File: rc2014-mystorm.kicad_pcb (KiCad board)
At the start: 2 copper layers, 100 x 50 mm, 15 parts, among them J1 CONN_02X06, J2 CONN_02X06, J3 CONN_02X06, J4 CONN_02X06, J6 CONN_02X06, J7 CONN_01X06, P1 RC2014 BUS, U1 SN74LVCC3245A, U2 SN74LVCC3245A, U3 SN74LVCC3245A, U4 SN74LVCC3245A

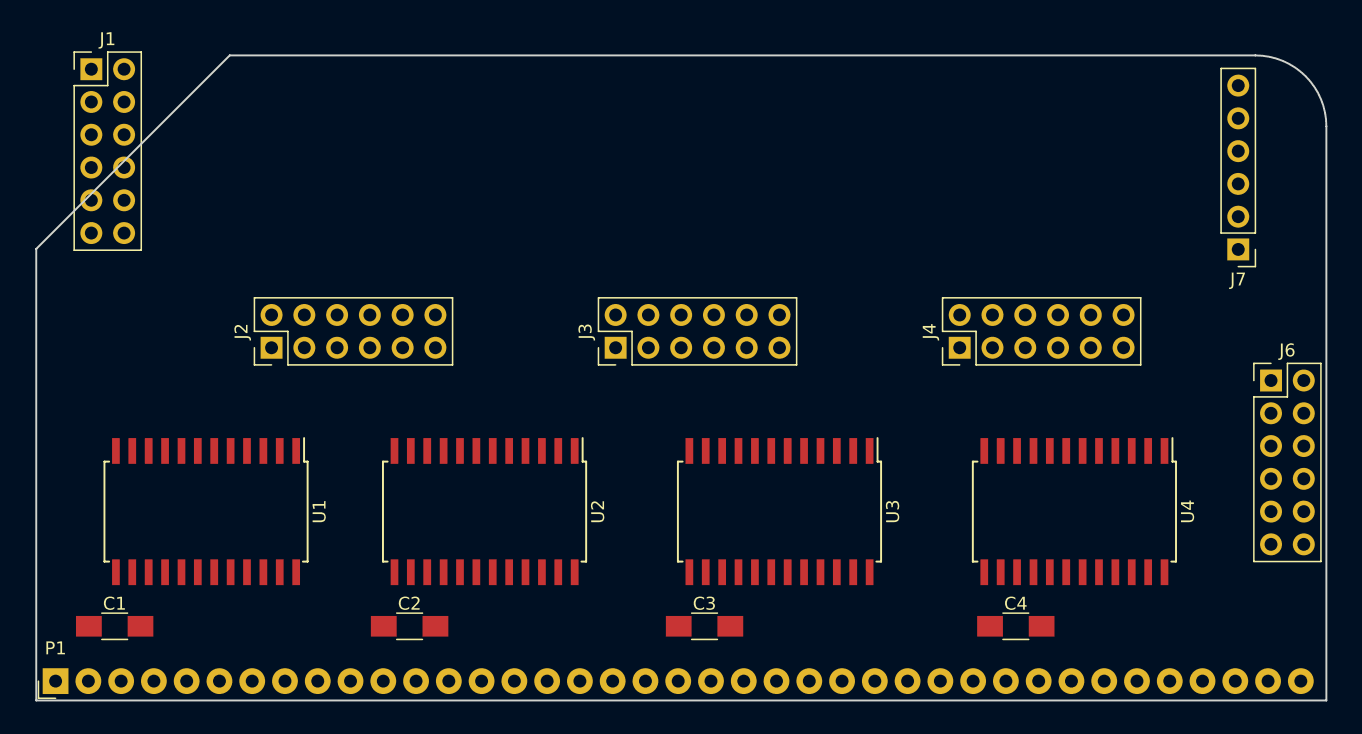
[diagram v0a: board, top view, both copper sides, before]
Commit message: further SMT WIP
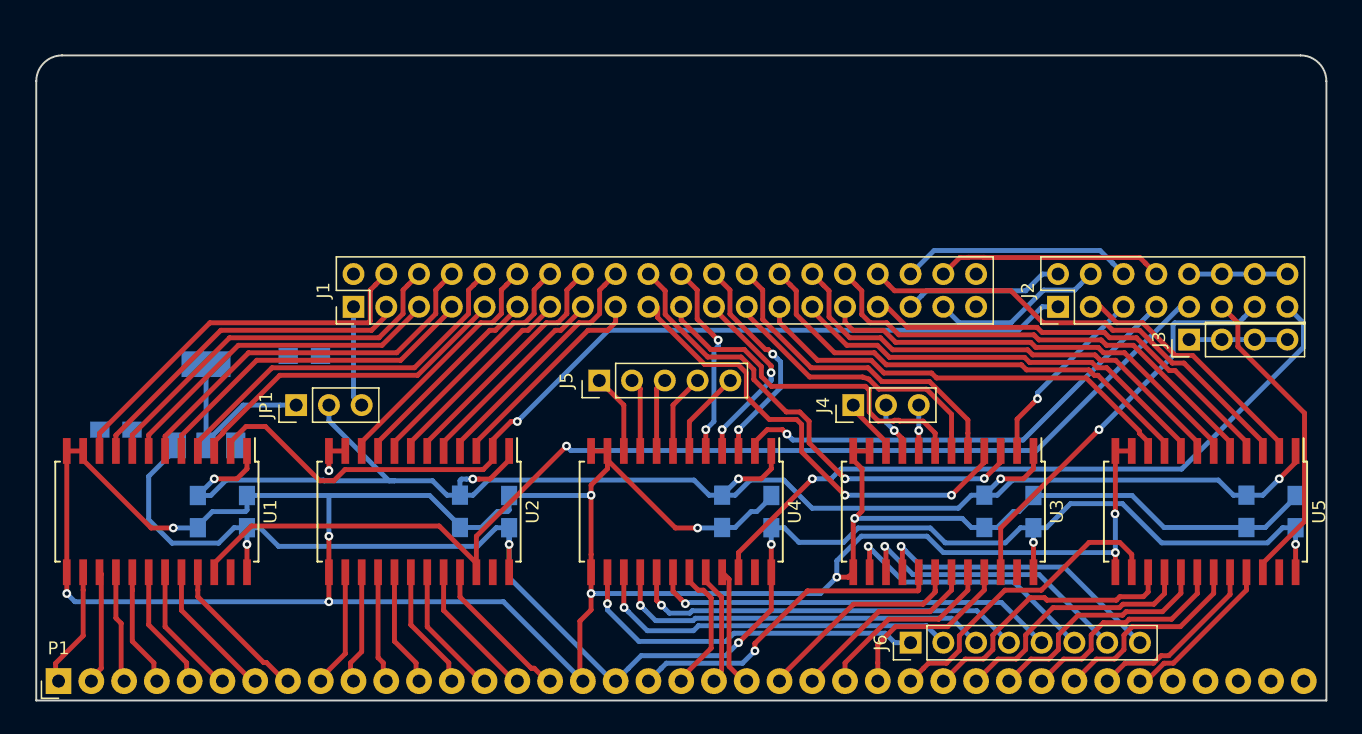
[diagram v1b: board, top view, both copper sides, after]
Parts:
- removed J7: CONN_01X06, Pin_Headers:Pin_Header_Straight_1x06_Pitch2.54mm
- added C10: C, Capacitors_SMD:C_0805_HandSoldering, B.Cu at (117.5, 149.9)
- added C11: C, Capacitors_SMD:C_0805_HandSoldering, B.Cu at (137.8, 149.9)
- added C12: C, Capacitors_SMD:C_0805_HandSoldering, B.Cu at (158.1, 149.9)
- added C5: C, Capacitors_SMD:C_0805_HandSoldering, B.Cu at (113.7, 149.8)
- added C6: C, Capacitors_SMD:C_0805_HandSoldering, B.Cu at (134.0, 149.8)
- added C7: C, Capacitors_SMD:C_0805_HandSoldering, B.Cu at (154.3, 149.8)
- added C8: C, Capacitors_SMD:C_0805_HandSoldering, B.Cu at (76.8, 149.9)
- added C9: C, Capacitors_SMD:C_0805_HandSoldering, B.Cu at (97.2, 149.9)
- added J5: Conn_01x05, Pin_Headers:Pin_Header_Straight_1x05_Pitch2.54mm, F.Cu at (104.1, 139.7)
- added JP1: Ext Power, Pin_Headers:Pin_Header_Straight_1x03_Pitch2.54mm, F.Cu at (80.6, 141.6)
- added U5: SN74LVCC3245A, Housings_SOIC:SOIC-24W_7.5x15.4mm_Pitch1.27mm, F.Cu at (151.1, 149.9)
- added U6: LM1117-3.3, TO_SOT_Packages_SMD:SOT-223-3_TabPin2, B.Cu at (73.7, 141.6)
- C1, C2: value C -> CP_Small; footprint Capacitors_SMD:C_1206_HandSoldering -> Capacitors_SMD:C_0805_HandSoldering; moved to B.Cu
- C3, C4: footprint Capacitors_SMD:C_1206_HandSoldering -> Capacitors_SMD:C_0805_HandSoldering; moved to B.Cu
- J1: value CONN_02X06 -> FPGA connection; footprint Pin_Headers:Pin_Header_Straight_2x06_Pitch2.54mm -> Pin_Headers:Pin_Header_Straight_2x20_Pitch2.54mm
- J2: value CONN_02X06 -> Config; footprint Pin_Headers:Pin_Header_Straight_2x06_Pitch2.54mm -> Pin_Headers:Pin_Header_Straight_2x08_Pitch2.54mm
- J3: value CONN_02X06 -> Conn_01x05; footprint Pin_Headers:Pin_Header_Straight_2x06_Pitch2.54mm -> Pin_Headers:Pin_Header_Straight_1x04_Pitch2.54mm
- J4: value CONN_02X06 -> Conn_01x03; footprint Pin_Headers:Pin_Header_Straight_2x06_Pitch2.54mm -> Pin_Headers:Pin_Header_Straight_1x03_Pitch2.54mm
- J6: value CONN_02X06 -> Extra; footprint Pin_Headers:Pin_Header_Straight_2x06_Pitch2.54mm -> Pin_Headers:Pin_Header_Straight_1x08_Pitch2.54mm
- moved J2 61.0 mm to (139.7, 134.0)
- moved J3 44.5 mm to (149.9, 136.5)
- moved C4 44.0 mm to (93.3, 149.8), turned to 270 degrees
- moved C3 40.3 mm to (73.0, 149.9), turned to 270 degrees
- moved J6 34.5 mm to (128.3, 160.0), turned to 90 degrees
- moved U4 30.5 mm to (110.5, 149.9)
- moved J1 27.4 mm to (85.1, 134.0), turned to 90 degrees
- moved C2 22.5 mm to (81.3, 137.8)
- moved C1 15.2 mm to (66.7, 143.5)
- moved U3 12.7 mm to (130.8, 149.9)
- moved J4 9.38 mm to (123.8, 141.6)
- moved U2 5.08 mm to (90.2, 149.9)
- moved U1 3.81 mm to (69.8, 149.9)
- moved P1 0.23 mm to (62.2, 163.0)
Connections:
- C1 pad 1: (no net) -> +5V
- C2 pad 1: (no net) -> Net-(C2-Pad1)
- C2 pad 2: (no net) -> GND
- C3 pad 1: (no net) -> +3V3
- C3 pad 2: (no net) -> GND
- C4 pad 1: (no net) -> +3V3
- C4 pad 2: (no net) -> GND
- J1 pad 1: GND -> /FPGA_VCC
- J1 pad 10: /A11LV -> /A9LV
- J1 pad 11: /A8LV -> /A6LV
- J1 pad 12: /A9LV -> /A7LV
- J1 pad 3: +3V3 -> /A14LV
- J1 pad 4: +3V3 -> /A15LV
- J1 pad 5: /A14LV -> /A12LV
- J1 pad 6: /A15LV -> /A13LV
- J1 pad 7: /A12LV -> /A10LV
- J1 pad 8: /A13LV -> /A11LV
- J1 pad 9: /A10LV -> /A8LV
- J2 pad 1: +3V3 -> /ADDR_DIR
- J2 pad 10: /A3LV -> GND
- J2 pad 11: /A0LV -> /DATA_OE
- J2 pad 12: /A1LV -> GND
- J2 pad 2: +3V3 -> /GPIO1
- J2 pad 3: GND -> /DATA_DIR
- J2 pad 4: GND -> /GPIO2
- J2 pad 5: /A6LV -> /SIG_DIR
- J2 pad 6: /A7LV -> /GPIO3
- J2 pad 7: /A4LV -> /SIG2_DIR
- J2 pad 8: /A5LV -> /GPIO4
- J2 pad 9: /A2LV -> /ADDR_OE
- J3 pad 3: GND -> +3V3
- J3 pad 4: GND -> +3V3
- J4 pad 1: /ADDR_DIR -> /EX3LV
- J4 pad 2: (no net) -> /EX2LV
- J4 pad 3: /DATA_DIR -> /EX1LV
- J6 pad 1: +3V3 -> /EX8
- J6 pad 2: +3V3 -> /EX7
- J6 pad 3: GND -> /EX6
- J6 pad 4: GND -> /EX5
- J6 pad 5: /D0LV -> /EX4
- J6 pad 6: /D1LV -> /EX3
- J6 pad 7: /D2LV -> /EX2
- J6 pad 8: /D3LV -> /EX1
- U1 pad 10: /A8LV -> /A15LV
- U1 pad 3: /A15LV -> /A8LV
- U1 pad 4: /A14LV -> /A9LV
- U1 pad 5: /A13LV -> /A10LV
- U1 pad 6: /A12LV -> /A11LV
- U1 pad 7: /A11LV -> /A12LV
- U1 pad 8: /A10LV -> /A13LV
- U1 pad 9: /A9LV -> /A14LV
- U2 pad 10: /A0LV -> /A7LV
- U2 pad 3: /A7LV -> /A0LV
- U2 pad 4: /A6LV -> /A1LV
- U2 pad 5: /A5LV -> /A2LV
- U2 pad 6: /A4LV -> /A3LV
- U2 pad 7: /A3LV -> /A4LV
- U2 pad 8: /A2LV -> /A5LV
- U2 pad 9: /A1LV -> /A6LV
- U3 pad 10: //IORQLV -> /EX3LV
- U3 pad 14: /M1 -> /EX3
- U3 pad 15: //RESET -> /EX2
- U3 pad 16: /CLK -> /EX1
- U3 pad 17: /INT -> /M1
- U3 pad 3: /M1LV -> //IORQLV
- U3 pad 4: //RESETLV -> //RDLV
- U3 pad 5: /CLKLV -> //WRLV
- U3 pad 6: /INTLV -> /MREQLV
- U3 pad 7: /MREQLV -> /M1LV
- U3 pad 8: //WRLV -> /EX1LV
- U3 pad 9: //RDLV -> /EX2LV
- U4 pad 10: /D7LV -> /EX8LV
- U4 pad 14: /D0 -> /EX8
- U4 pad 15: /D1 -> /EX7
- U4 pad 16: /D2 -> /EX6
- U4 pad 17: /D3 -> /EX5
- U4 pad 18: /D4 -> /EX4
- U4 pad 19: /D5 -> //RESET
- U4 pad 2: /DATA_DIR -> /SIG2_DIR
- U4 pad 20: /D6 -> /CLK
- U4 pad 21: /D7 -> /INT
- U4 pad 22: /DATA_OE -> /SIG2_OE
- U4 pad 3: /D0LV -> /INTLV
- U4 pad 4: /D1LV -> /CLKLV
- U4 pad 5: /D2LV -> //RESETLV
- U4 pad 6: /D3LV -> /EX4LV
- U4 pad 7: /D4LV -> /EX5LV
- U4 pad 8: /D5LV -> /EX6LV
- U4 pad 9: /D6LV -> /EX7LV
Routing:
- net GND: track 0.00 -> 263.6 mm, vias 0 -> 12
- net +5V: track 0.00 -> 132.2 mm, vias 0 -> 6
- net +3V3: track 0.00 -> 132.1 mm, vias 0 -> 5
- net /ADDR_OE: track 0.00 -> 89.8 mm, vias 0 -> 1
- net /ADDR_DIR: track 0.00 -> 74.3 mm, vias 0 -> 1
- net /SIG2_OE: track 0.00 -> 55.6 mm, vias 0 -> 1
- net //IORQLV: track 0.00 -> 38.5 mm, vias 0 -> 2
- net /D3LV: track 0.00 -> 37.1 mm
- net /D1LV: track 0.00 -> 37.0 mm
- net /D5LV: track 0.00 -> 37.0 mm
- net /SIG2_DIR: track 0.00 -> 36.8 mm, vias 0 -> 1
- net //RDLV: track 0.00 -> 36.8 mm, vias 0 -> 2
- net /D7LV: track 0.00 -> 35.9 mm
- net /D0LV: track 0.00 -> 34.4 mm
- net /D4LV: track 0.00 -> 34.3 mm
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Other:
- outline, holes or cut-outs redrawn
- net class Default: clearance 0.254 -> 0.2
- rule trace_clearance: 0.254 -> 0.2
- board text added: "A15"
- board text added: "github.com/electrified/rc2014-fpga"
- board text removed: "github.com/electrified/rc2014-ym2149"

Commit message: WIP
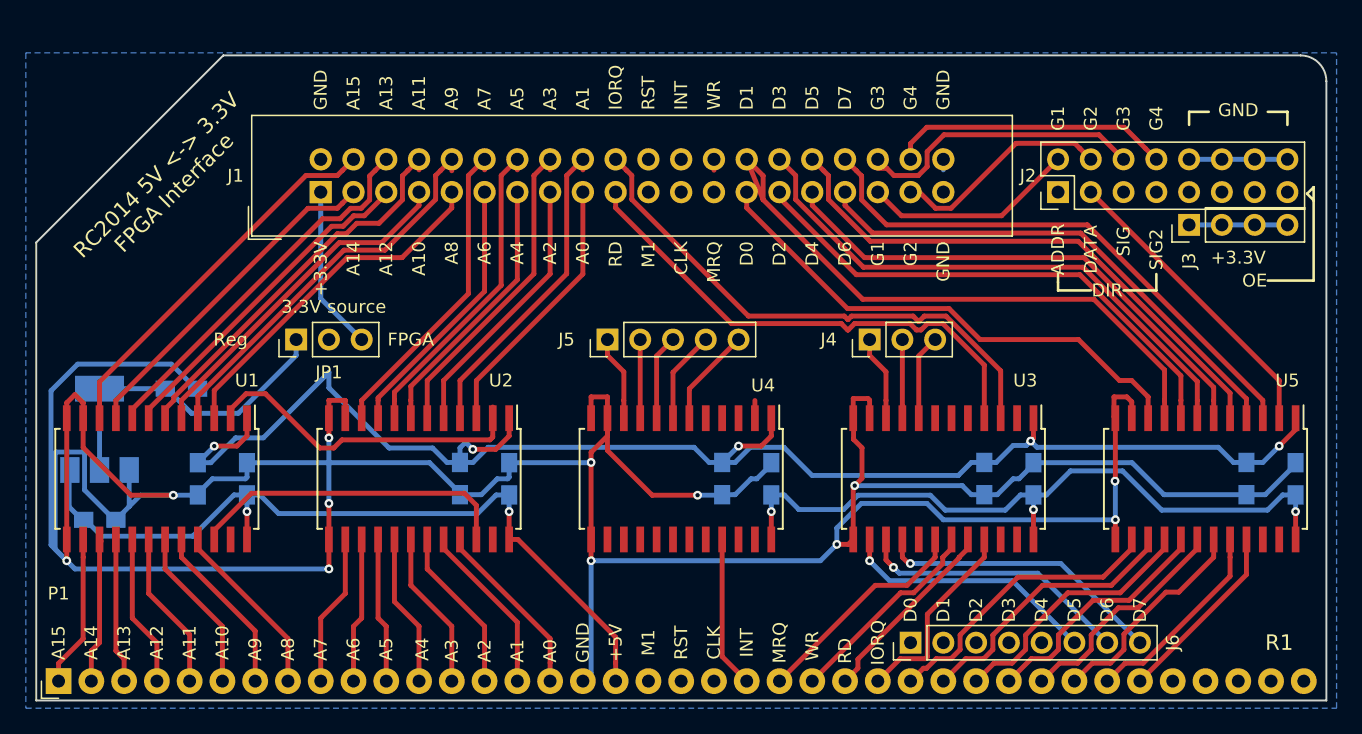
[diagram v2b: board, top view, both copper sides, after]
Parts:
- added REF***: OSHW-Logo_7.5x8mm_SilkScreen, Symbols:OSHW-Logo_7.5x8mm_SilkScreen, B.Cu at (71.1, 125.7)
- J1: footprint Pin_Headers:Pin_Header_Straight_2x20_Pitch2.54mm -> Connectors_IDC:IDC-Header_2x20_Pitch2.54mm_Straight
- moved C2 9.86 mm to (71.8, 140.3)
- moved J1 9.25 mm to (82.5, 125.1)
- moved J2 8.89 mm to (139.7, 125.1)
- moved J3 8.89 mm to (149.9, 127.6)
- moved U6 8.47 mm to (65.4, 143.5)
- moved C1 7.10 mm to (65.4, 150.5)
- moved J4 5.24 mm to (125.1, 136.5)
- moved JP1 5.08 mm to (80.6, 136.5)
- moved J5 3.24 mm to (104.8, 136.5)
- moved C10 2.54 mm to (117.5, 147.3)
- moved C11 2.54 mm to (137.8, 147.3)
- moved C12 2.54 mm to (158.1, 147.3)
- moved C3 2.54 mm to (73.0, 147.3)
- moved C8 2.54 mm to (76.8, 147.3)
- moved C9 2.54 mm to (97.2, 147.3)
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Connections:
- J1 pad 39: /FPGA_VCC -> GND
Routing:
- net /ADDR_OE: track 89.8 -> 25.3 mm, vias 1 -> 0
- net /SIG2_OE: track 55.6 -> 0.00 mm, vias 1 -> 0
- net GND: track 263.6 -> 315.0 mm
- net /ADDR_DIR: track 74.3 -> 26.6 mm, vias 1 -> 0
- net /SIG2_DIR: track 36.8 -> 1.37 mm, vias 1 -> 0
- net /EX4: track 31.8 -> 0.00 mm, vias 1 -> 0
- net /SIG_OE: track 31.6 -> 0.00 mm, vias 1 -> 0
- net /EX5: track 31.0 -> 0.00 mm, vias 1 -> 0
- net /EX6: track 29.9 -> 0.00 mm, vias 1 -> 0
- net /EX7: track 28.9 -> 0.00 mm, vias 1 -> 0
- net /EX8: track 28.0 -> 0.00 mm, vias 1 -> 0
- net /M1LV: track 27.2 -> 0.00 mm
- net /M1: track 26.3 -> 0.00 mm, vias 1 -> 0
- net //WRLV: track 25.6 -> 0.14 mm
- net /DATA_OE: track 24.6 -> 0.70 mm
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- added copper zone on B.Cu, net GND
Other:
- outline, holes or cut-outs redrawn
- net class IO: clearance 0.254 -> 0.2
- net class analogue: clearance 0.254 -> 0.2
- net class gnd: clearance 0.254 -> 0.2
- net class vcc: clearance 0.254 -> 0.2
- board text added: "+3.3V"
- board text added: "+5V"
- board text added: "3.3V source"
- board text added: "A0"
- board text added: "A1"
- board text added: "A10"
- board text added: "A11"
- board text added: "A12"
- board text added: "A13"
- board text added: "A14"
- board text added: "A2"
- board text added: "A3"
- board text added: "A4"
- board text added: "A5"
- board text added: "A6"
- board text added: "A7"
- board text added: "A8"
- board text added: "A9"
- board text added: "ADDR"
- board text added: "CLK"
- board text added: "D0"
- board text added: "D1"
- board text added: "D2"
- board text added: "D3"
- board text added: "D4"
- board text added: "D5"
- board text added: "D6"
- board text added: "D7"
- board text added: "DATA"
- board text added: "DIR"
- board text added: "FPGA"
- board text added: "G1"
- board text added: "G2"
- board text added: "G3"
- board text added: "G4"
- board text added: "GND"
- board text added: "INT"
- board text added: "IORQ"
- board text added: "M1"
- board text added: "MRQ"
- board text added: "OE"
- board text added: "R1"
- board text added: "RC2014 5V <-> 3.3V FPGA Interface"
- board text added: "RD"
- board text added: "RST"
- board text added: "Reg"
- board text added: "SIG"
- board text added: "SIG2"
- board text added: "WR"
- board text added: "github.com/electrified/rc2014-fpga-interface"
- board text removed: "github.com/electrified/rc2014-fpga"
